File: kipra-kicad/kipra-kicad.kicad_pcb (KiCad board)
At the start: 2 copper layers, 128.2 x 134.8 mm, 52 parts

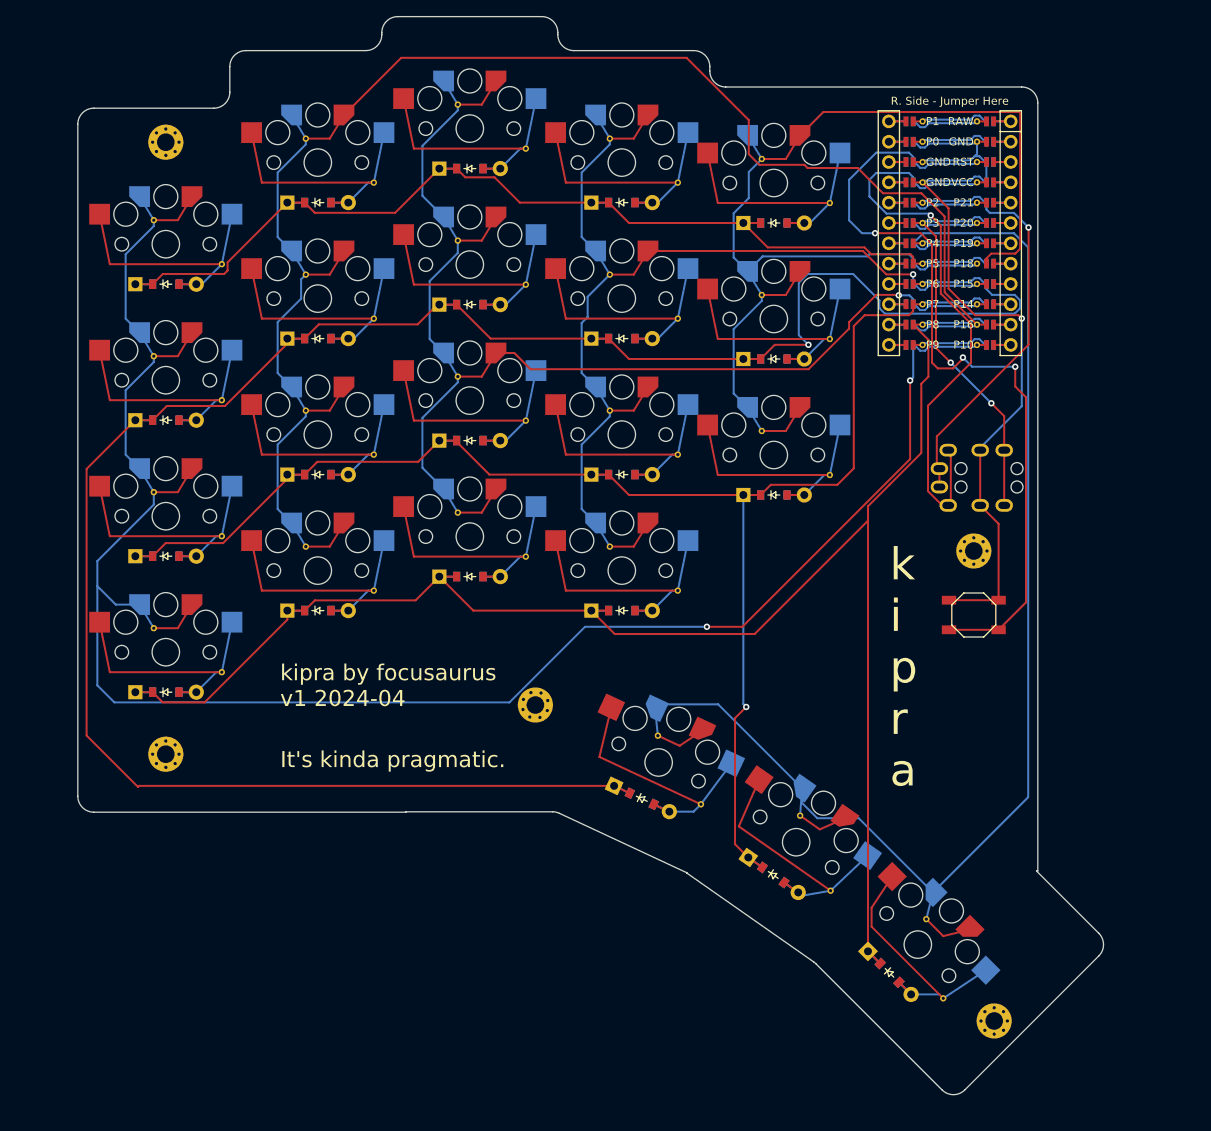
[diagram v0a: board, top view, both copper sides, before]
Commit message: DRC passes
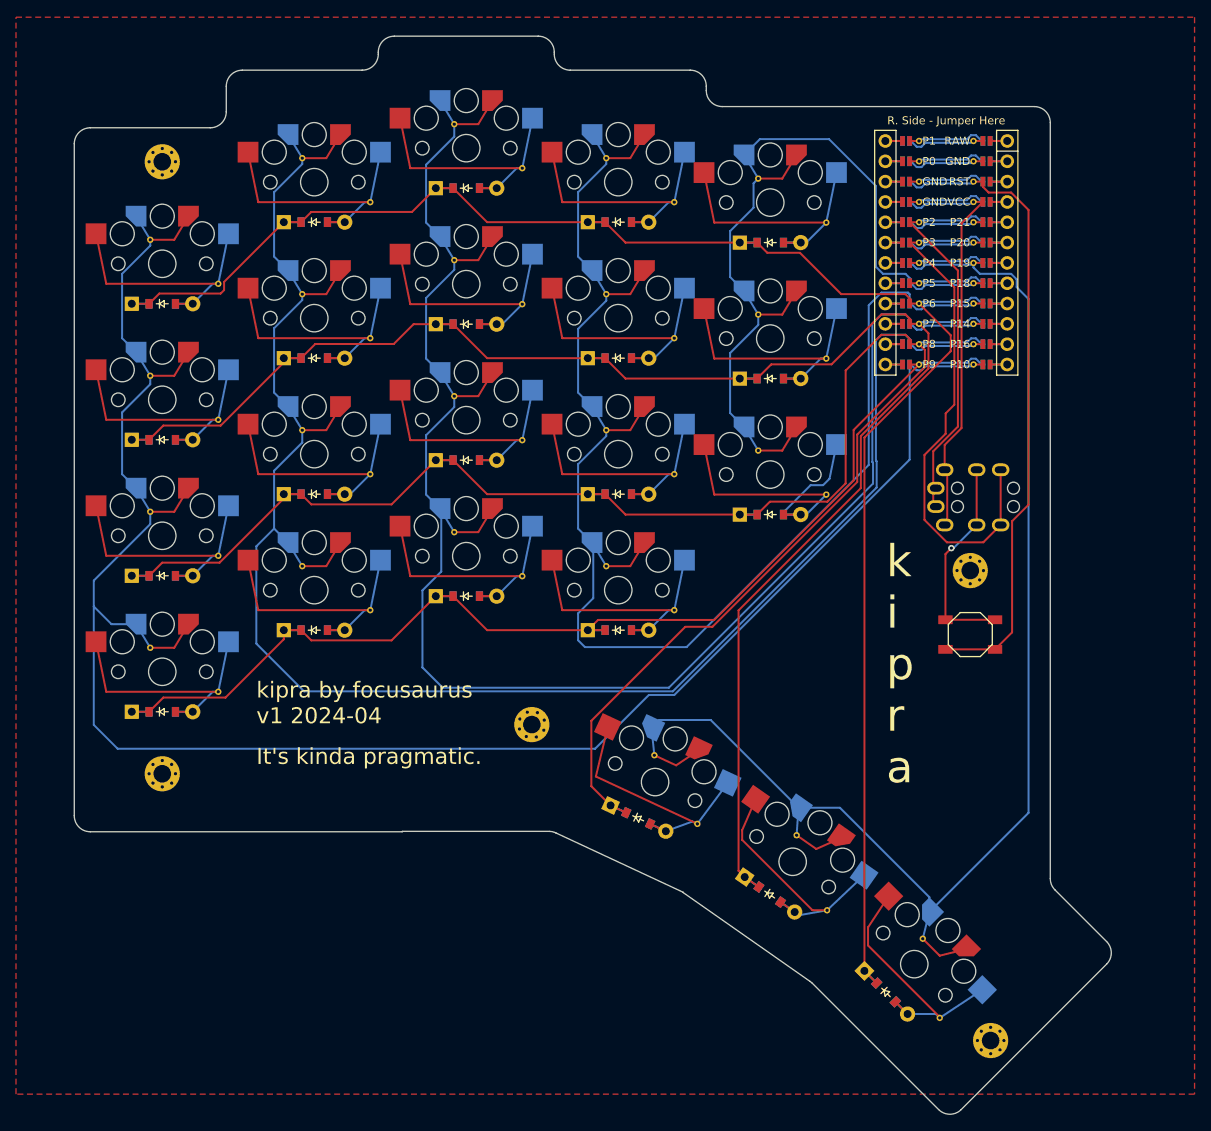
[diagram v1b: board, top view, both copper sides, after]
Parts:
- moved D11 2.49 mm to (137.6, 56.2)
- moved TRRS1 2.49 mm to (207.6, 79.0)
- moved S20 2.49 mm to (193.6, 136.2)
- moved S21 2.49 mm to (178.4, 123.4)
- moved D21 2.49 mm to (175.5, 127.4)
- moved S18 2.49 mm to (175.6, 58.0)
- moved D12 2.49 mm to (137.6, 39.2)
- moved S19 2.49 mm to (175.6, 41.0)
- moved S3 2.49 mm to (99.6, 65.6)
- moved S17 2.49 mm to (175.6, 75.0)
- moved D17 2.49 mm to (175.6, 80.0)
- moved D2 2.49 mm to (99.6, 87.6)
- moved _1 2.49 mm to (99.6, 112.4)
- moved D16 2.49 mm to (156.6, 43.4)
- moved S4 2.49 mm to (99.6, 48.6)
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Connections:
- D1 pad 1: P8 -> P9
- D10 pad 1: P7 -> P8
- D11 pad 1: P6 -> P7
- D12 pad 1: P5 -> P6
- D13 pad 1: P8 -> P9
- D14 pad 1: P7 -> P8
- D15 pad 1: P6 -> P7
- D16 pad 1: P5 -> P6
- D17 pad 1: P7 -> P8
- D18 pad 1: P6 -> P7
- D19 pad 1: P5 -> P6
- D2 pad 1: P7 -> P8
- D20 pad 1: P8 -> P6
- D22 pad 1: P6 -> P8
- D3 pad 1: P6 -> P7
- D4 pad 1: P5 -> P6
- D5 pad 1: P8 -> P9
- D6 pad 1: P7 -> P8
- D7 pad 1: P6 -> P7
- D8 pad 1: P5 -> P6
- D9 pad 1: P8 -> P9
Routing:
- net P9: track 9.29 -> 145.8 mm
- net P5: track 132.6 -> 9.64 mm
- net P14: track 157.3 -> 212.8 mm, vias 1 -> 0
- net P15: track 133.1 -> 184.0 mm, vias 1 -> 0
- net P6: track 274.8 -> 224.5 mm, vias 1 -> 0
- net GND: track 102.2 -> 55.6 mm
- net P18: track 143.8 -> 107.0 mm
- net P16: track 201.5 -> 227.6 mm
- net RST: track 103.9 -> 80.0 mm, vias 3 -> 0
- net VCC: track 75.9 -> 52.3 mm, vias 1 -> 0
- net P3: track 48.8 -> 66.7 mm, vias 2 -> 0
- net P7: track 198.4 -> 215.1 mm, vias 1 -> 0
- net P8: track 219.2 -> 228.8 mm
- net P19: track 185.9 -> 176.8 mm
- net inner_two: track 35.3 -> 41.1 mm
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- added copper zone on F.Cu, net GND
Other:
- board size 128.2 x 134.8 mm -> 129.6 x 134.8 mm
- board text removed: "P2"
